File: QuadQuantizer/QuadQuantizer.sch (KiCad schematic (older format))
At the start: 70 parts, among them J1 OLED, J2 R_ENC, J3 CV_IN, J4 CV_OUT, J5 TR_OUT, J6 POWER, M1 RP2040zero, SW1 Rotary_Encoder_Switch, SW2 RESET, U1 24LC04, U2 MAX5715BAUD, U3 TL074, U4 TL074

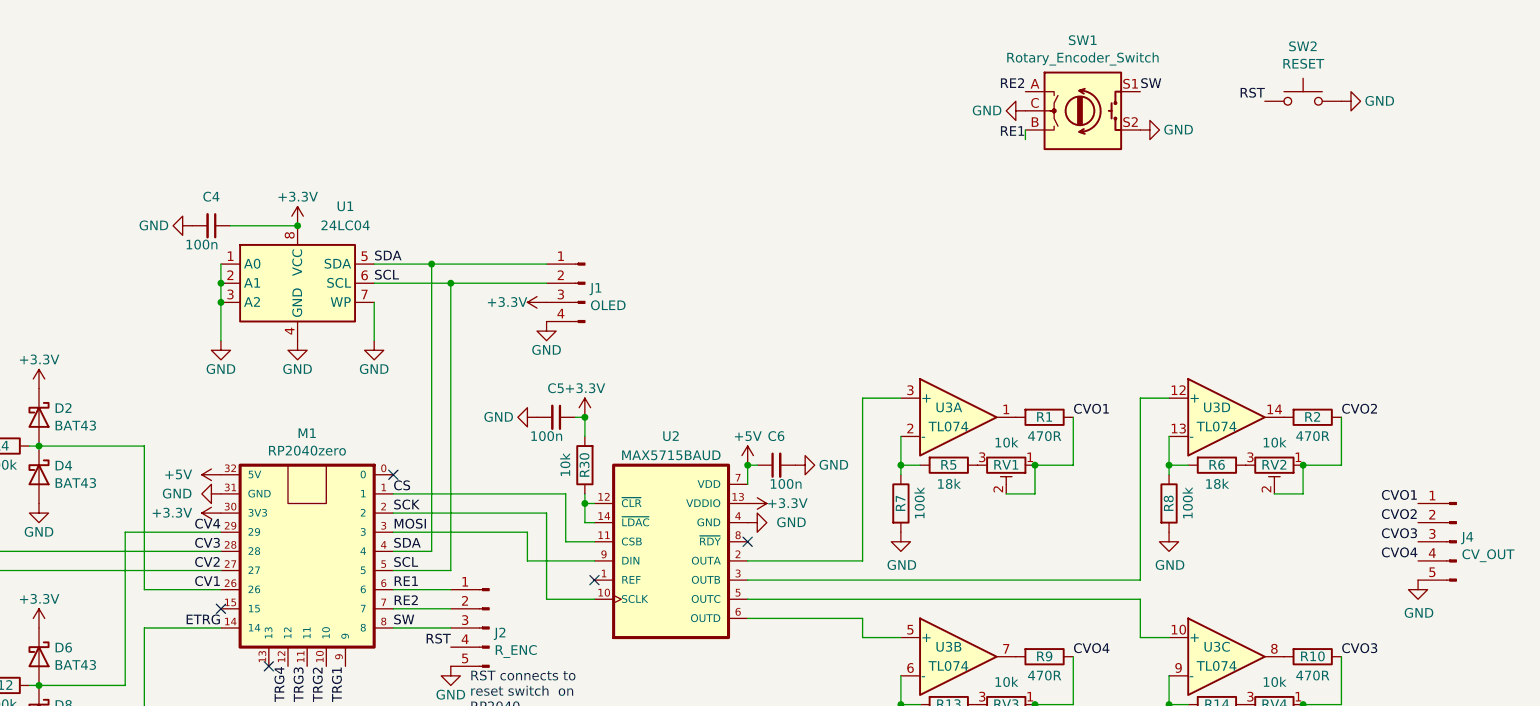
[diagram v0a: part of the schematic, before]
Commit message: Add files via upload
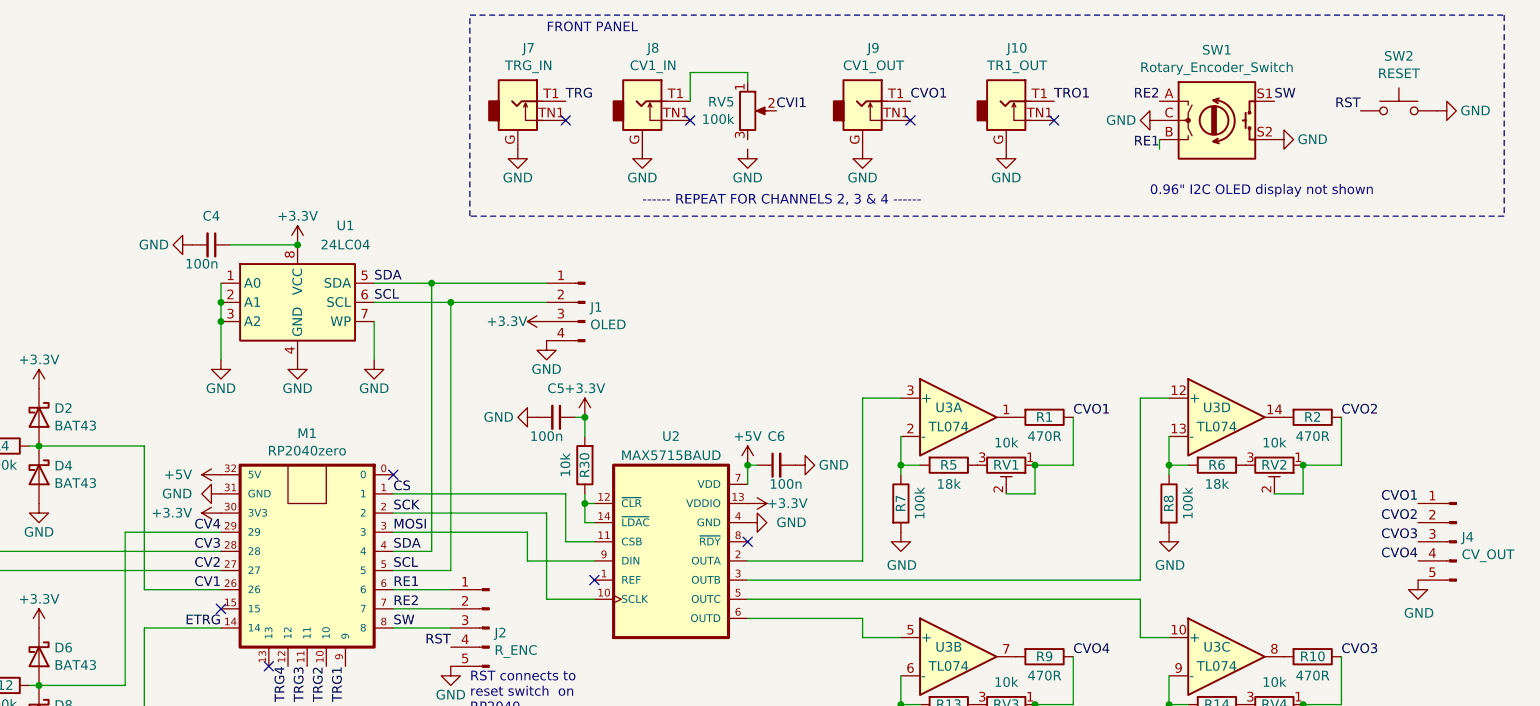
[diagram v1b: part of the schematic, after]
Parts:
- added J10: TR1_OUT, symbol CGE_symbols:AudioJack_Ground_Switch
- added J7: TRG_IN, symbol CGE_symbols:AudioJack_Ground_Switch
- added J8: CV1_IN, symbol CGE_symbols:AudioJack_Ground_Switch
- added J9: CV1_OUT, symbol CGE_symbols:AudioJack_Ground_Switch
- added RV5: 100k, symbol Device:R_POT
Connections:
- net CVI1: now also RV5.2
- net CVO1: now also J9.T1
- net GND: now also J10.G, J7.G, J8.G, J9.G
- net TRG: now also J7.T1
- net TRO1: now also J10.T1
- new net: J8.T1, RV5.1
- no-connect marks 5 -> 9
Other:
- note added: "------ REPEAT FOR CHANNELS 2, 3 & 4 ------"
- note added: "0.96" I2C OLED display not shown"
- note added: "FRONT PANEL"
- moved on the sheet: C4, J1, SW1, SW2, U1
